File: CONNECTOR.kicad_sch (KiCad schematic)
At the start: 11 parts, among them J10 SWD, J2 SPI, J7 CONNECTOR

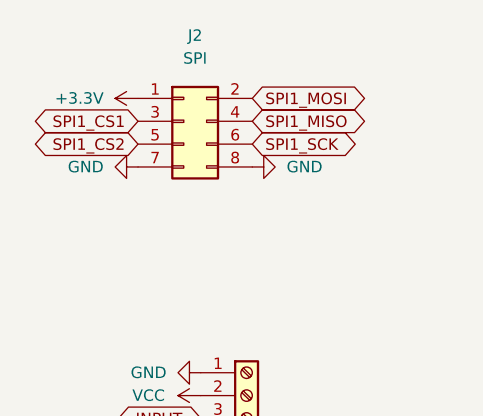
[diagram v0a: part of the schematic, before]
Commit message: Add files via upload
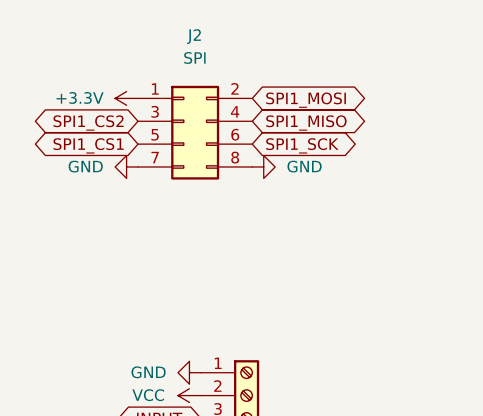
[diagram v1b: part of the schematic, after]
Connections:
- net SPI1_CS1: now also J2.5 (Pin_5); no longer J2.3 (Pin_3)
- net SPI1_CS2: now also J2.3 (Pin_3); no longer J2.5 (Pin_5)
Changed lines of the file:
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@@
 (kicad_sch (version 20211123) (generator eeschema)
   (paper "A5")
-  (global_label "SPI1_CS2" (shape bidirectional) (at 64.135 34.925 180) (fields_autoplaced)
+  (global_label "SPI1_CS2" (shape bidirectional) (at 64.135 32.385 180) (fields_autoplaced)
     (effects (font (size 1.27 1.27)) (justify right))
-    (property "Intersheet References" "${INTERSHEET_REFS}" (id 0) (at 52.7714 34.8456 0)
+    (property "Intersheet References" "${INTERSHEET_REFS}" (id 0) (at 52.7714 32.4644 0)
       (effects (font (size 1.27 1.27)) (justify right) hide)
     )
@@
     )
   )
-  (global_label "SPI1_CS1" (shape bidirectional) (at 64.135 32.385 180) (fields_autoplaced)
+  (global_label "SPI1_CS1" (shape bidirectional) (at 64.135 34.925 180) (fields_autoplaced)
     (effects (font (size 1.27 1.27)) (justify right))
-    (property "Intersheet References" "${INTERSHEET_REFS}" (id 0) (at 52.7714 32.3056 0)
+    (property "Intersheet References" "${INTERSHEET_REFS}" (id 0) (at 52.7714 35.0044 0)
       (effects (font (size 1.27 1.27)) (justify right) hide)
     )
